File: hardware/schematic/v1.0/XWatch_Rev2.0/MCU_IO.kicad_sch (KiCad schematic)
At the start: 12 parts, among them U1 STM32U5G9NJH6Q, U15 STM32U5A9BJY6QTR, X1 32.768KHZ, X2 16MHZ

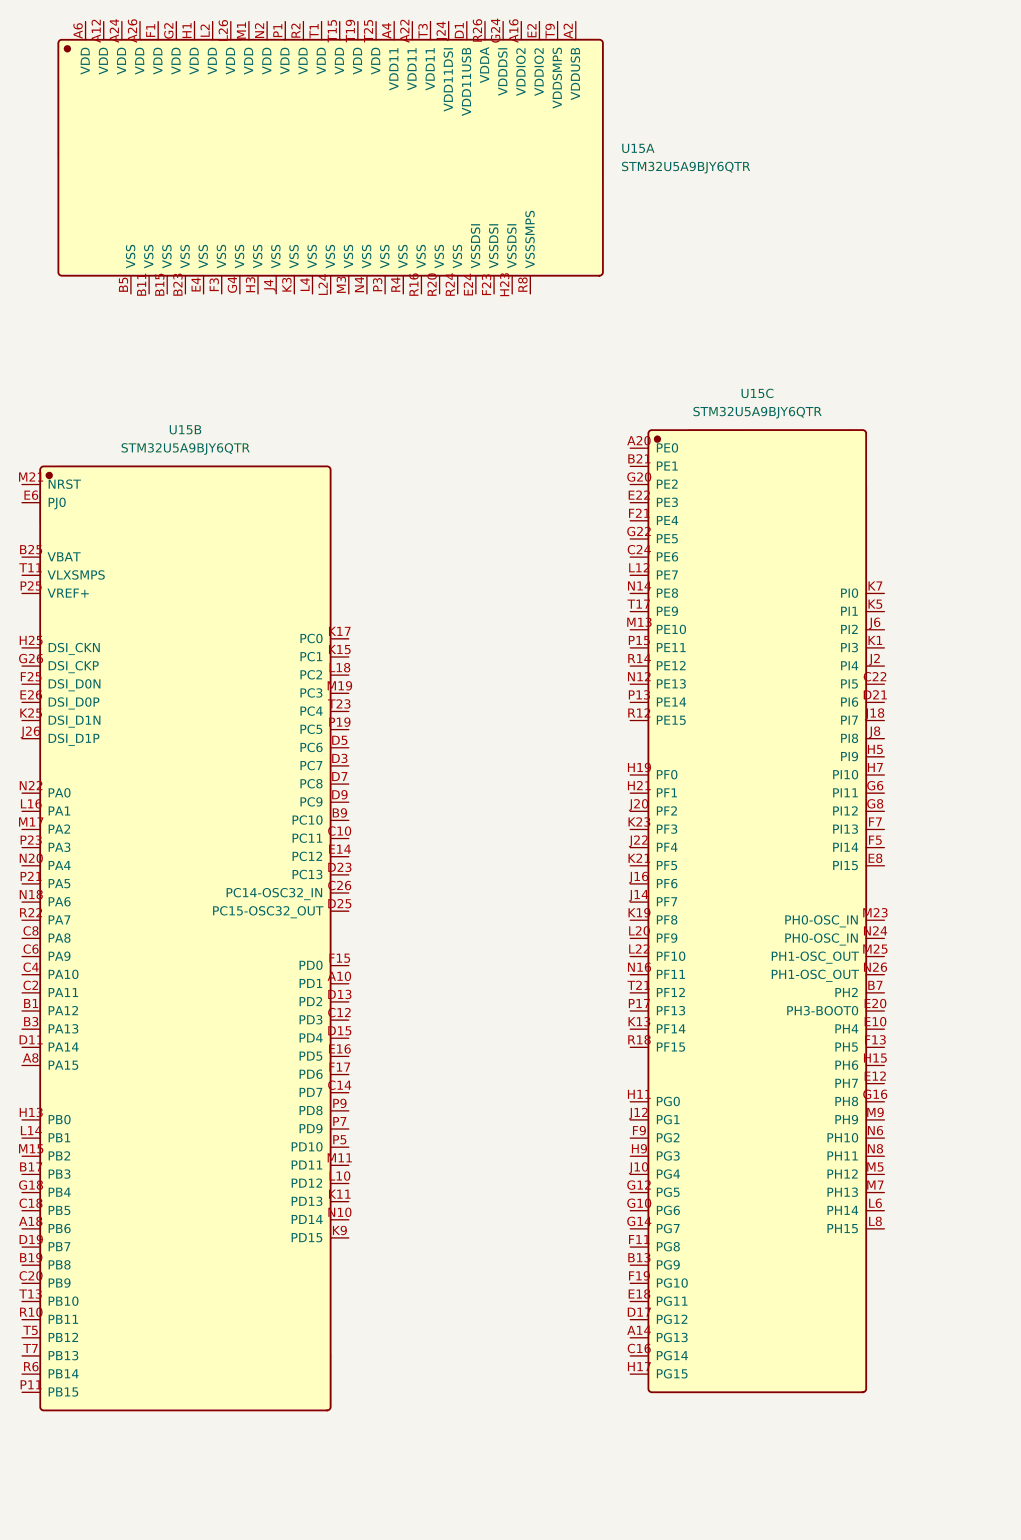
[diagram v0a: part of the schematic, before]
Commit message: add XWatch_Rev3.0
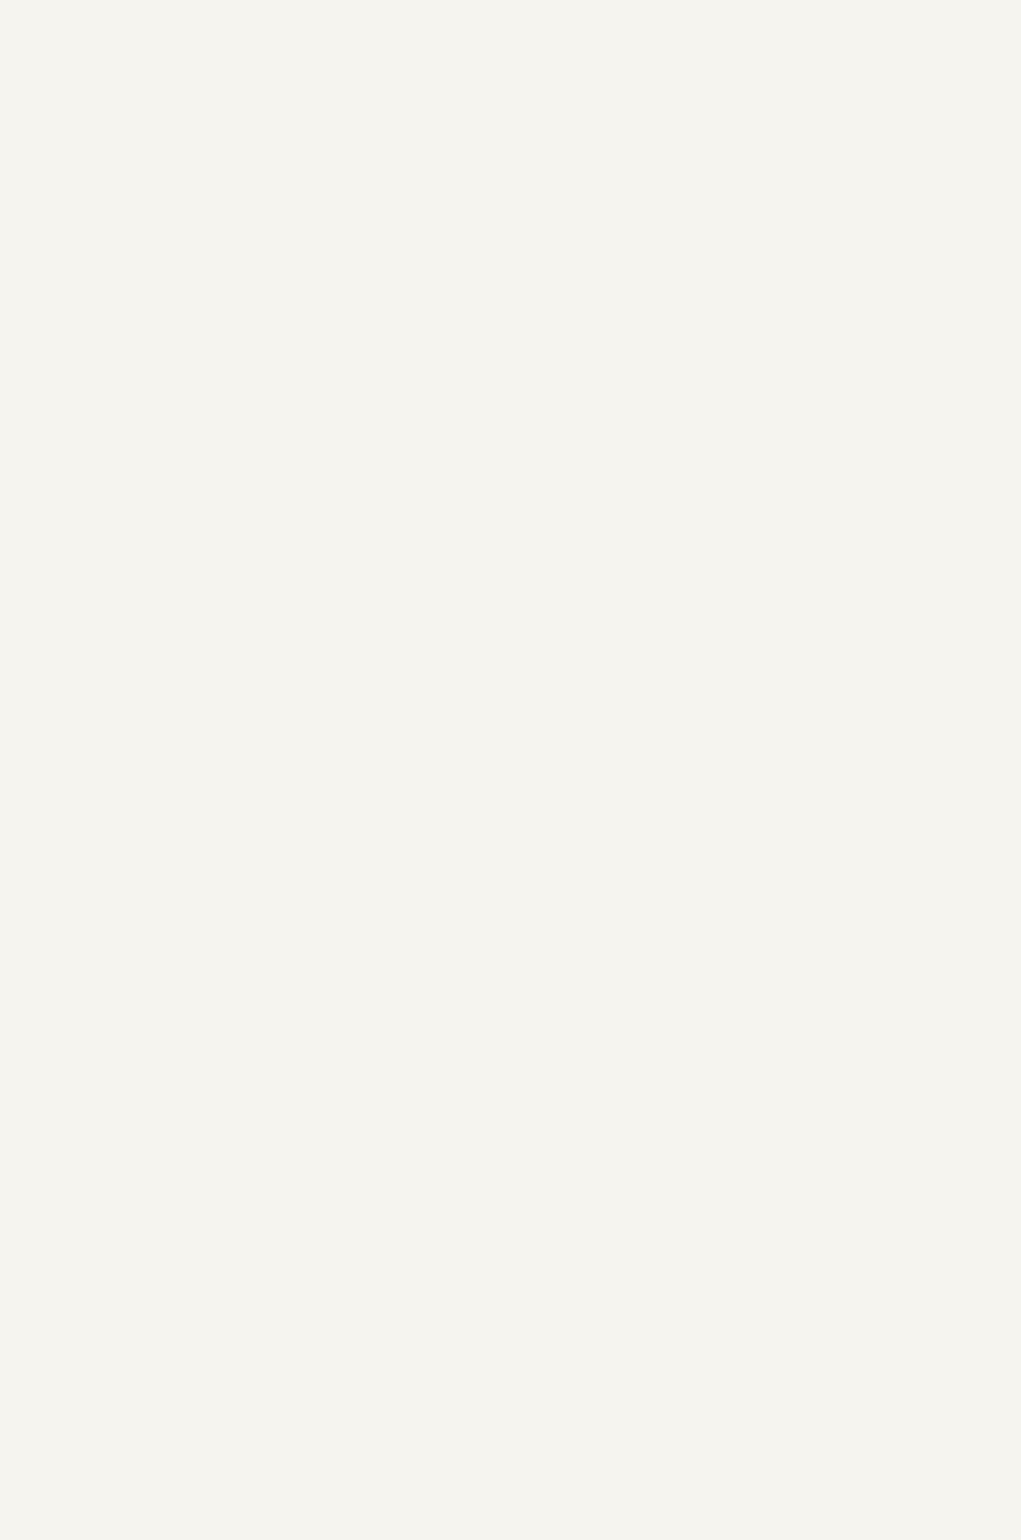
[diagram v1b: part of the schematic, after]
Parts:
- removed U15: STM32U5A9BJY6QTR, XWatch_Rev2.0:STM32U5A9BJY6QTR, symbol XWatch_Rev2.0:STM32U5A9BJY6QTR

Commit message: sch update
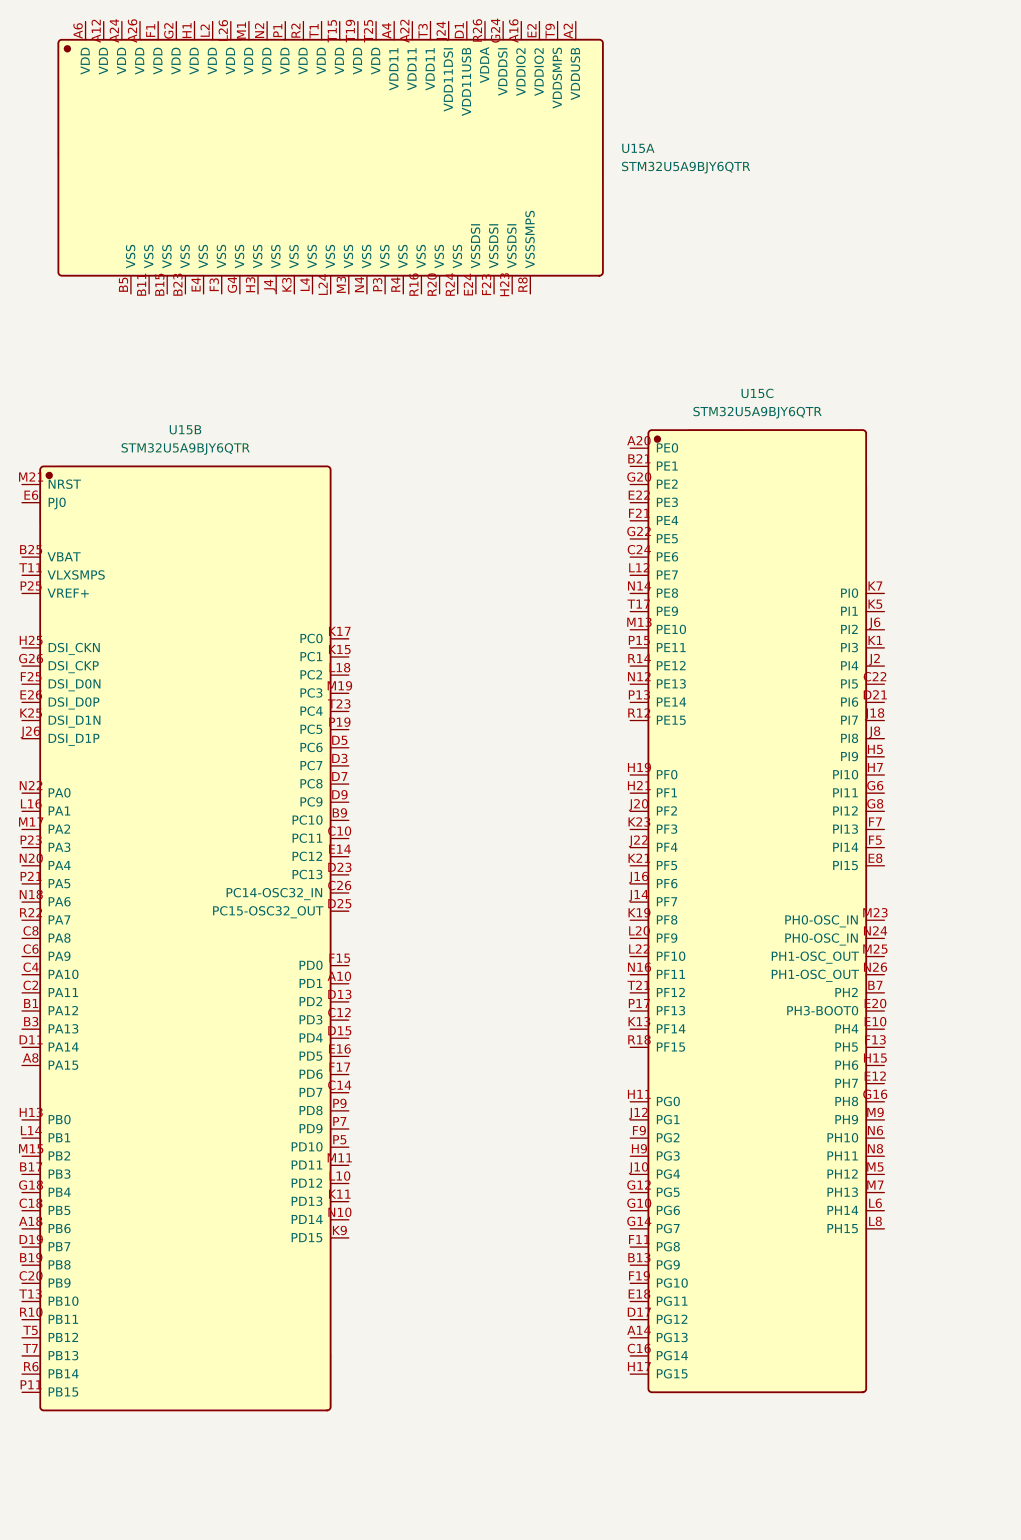
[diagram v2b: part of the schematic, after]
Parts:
- added U15: STM32U5A9BJY6QTR, XWatch_Rev2.0:STM32U5A9BJY6QTR, symbol XWatch_Rev2.0:STM32U5A9BJY6QTR
